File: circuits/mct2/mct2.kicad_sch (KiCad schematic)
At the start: 4 parts, among them J1 Bus_M.2_Socket_M, J2 Bus_M.2_Socket_E, U1 BQ25700A

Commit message: schem update July 19 2024
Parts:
- removed U1: BQ25700A, symbol mediacow:BQ25700A
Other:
- added sheet mct2_power (mct2_power.kicad_sch)
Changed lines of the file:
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@@
-		)
-	)
-	(wire
-		(pts
-			(xy 229.87 749.3) (xy 232.41 749.3)
-		)
-		(stroke
-			(width 0)
-			(type default)
 		)
 	)
@@
 		)
 	)
-	(global_label "PROCHOT"
-		(shape input)
-		(at 229.87 749.3 180)
-		(fields_autoplaced yes)
-		(effects
-			(font
-				(size 1.27 1.27)
-			)
-			(justify right)
-		)
-		(property "Intersheetrefs" "${INTERSHEET_REFS}"
-			(at 218.1157 749.3 0)
-			(effects
-				(font
-					(size 1.27 1.27)
-				)
-				(justify right)
-				(hide yes)
-			)
-		)
-	)
 	(global_label "AC_LRCLK"
 		(shape input)
@@
 				(justify left)
 				(hide yes)
-			)
-		)
-	)
-	(symbol
-		(lib_id "mediacow:BQ25700A")
-		(at 247.65 742.95 0)
-		(unit 1)
-		(exclude_from_sim no)
-		(in_bom yes)
-		(on_board yes)
-		(dnp no)
-		(property "Reference" "U1"
-			(at 236.22 720.344 0)
-			(effects
-				(font
-					(size 1.27 1.27)
-				)
-			)
-		)
-		(property "Value" "BQ25700A"
-			(at 243.332 720.344 0)
-			(effects
-				(font
-					(size 1.27 1.27)
-				)
-			)
-		)
-		(property "Footprint" ""
-			(at 241.3 727.71 0)
-			(effects
-				(font
-					(size 1.27 1.27)
-				)
-				(hide yes)
-			)
-		)
-		(property "Datasheet" ""
-			(at 241.3 727.71 0)
-			(effects
-				(font
-					(size 1.27 1.27)
-				)
-				(hide yes)
-			)
-		)
-		(property "Description" ""
-			(at 241.3 727.71 0)
-			(effects
-				(font
-					(size 1.27 1.27)
-				)
-				(hide yes)
-			)
-		)
-		(pin "32"
-		)
-		(pin "23"
-		)
-		(pin "25"
-		)
-		(pin "17"
-		)
-		(pin "22"
-		)
-		(pin "6"
-		)
-		(pin "31"
-		)
-		(pin "19"
-		)
-		(pin "29"
-		)
-		(pin "16"
-		)
-		(pin "26"
-		)
-		(pin "15"
-		)
-		(pin "1"
-		)
-		(pin "28"
-		)
-		(pin "11"
-		)
-		(pin "13"
-		)
-		(pin "9"
-		)
-		(pin "5"
-		)
-		(pin "12"
-		)
-		(pin "3"
-		)
-		(pin "8"
-		)
-		(pin "20"
-		)
-		(pin "21"
-		)
-		(pin "30"
-		)
-		(pin "4"
-		)
-		(pin "27"
-		)
-		(pin "10"
-		)
-		(pin "7"
-		)
-		(pin "2"
-		)
-		(pin "24"
-		)
-		(pin "18"
-		)
-		(pin "14"
-		)
-		(instances
-			(project "mct2"
-				(path "/0917e100-0497-47cd-9e32-3e43ad224d2b"
-					(reference "U1")
-					(unit 1)
-				)
 			)
 		)
@@
 				)
 			)
+		)
+	)
+	(sheet
+		(at 688.34 405.13)
+		(size 67.31 55.88)
+		(fields_autoplaced yes)
+		(stroke
+			(width 0.1524)
+			(type solid)
+		)
+		(fill
+			(color 0 0 0 0.0000)
+		)
+		(property "Sheetname" "mct2_power"
+			(at 688.34 404.4184 0)
+			(effects
+				(font
+					(size 1.27 1.27)
+				)
+				(justify left bottom)
+			)
+		)
+		(property "Sheetfile" "mct2_power.kicad_sch"
+			(at 688.34 461.5946 0)
+			(effects
+				(font
+					(size 1.27 1.27)
+				)
+				(justify left top)
+			)
+		)
+		(instances
+			(project "mct2"
+				(path "/0917e100-0497-47cd-9e32-3e43ad224d2b"
+					(page "3")
+				)
+			)

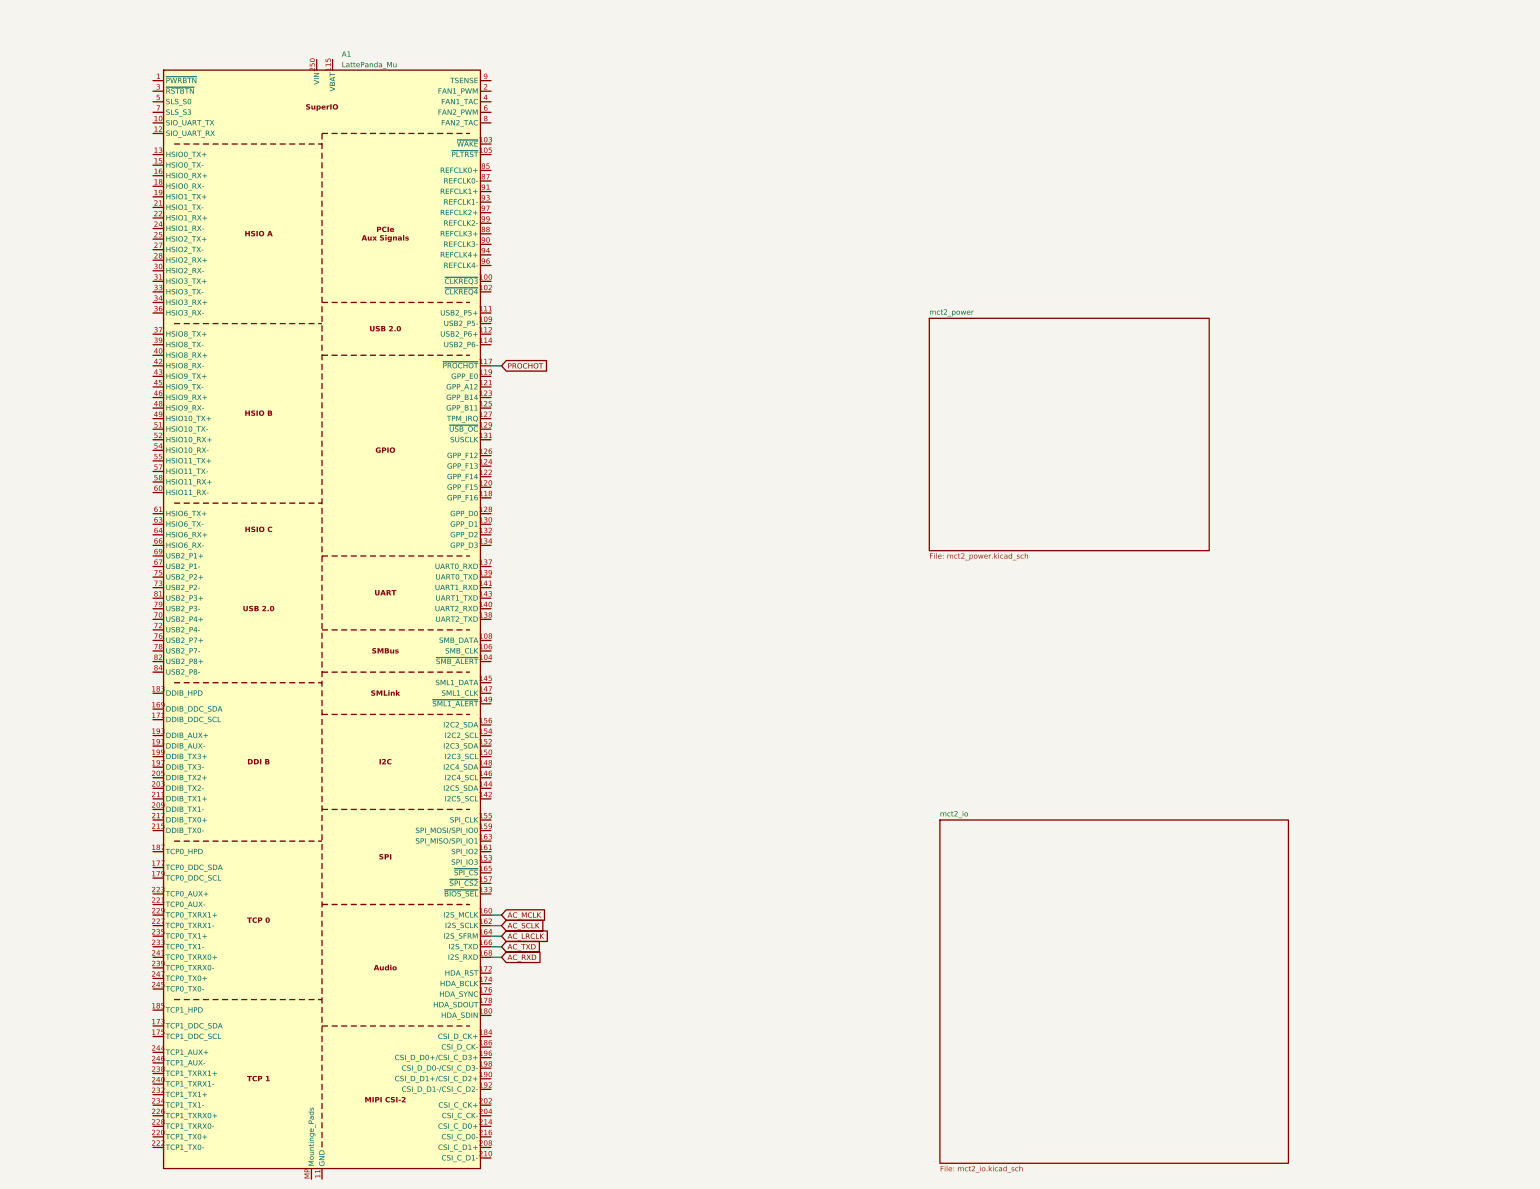
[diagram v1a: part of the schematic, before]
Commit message: July 21, 2024
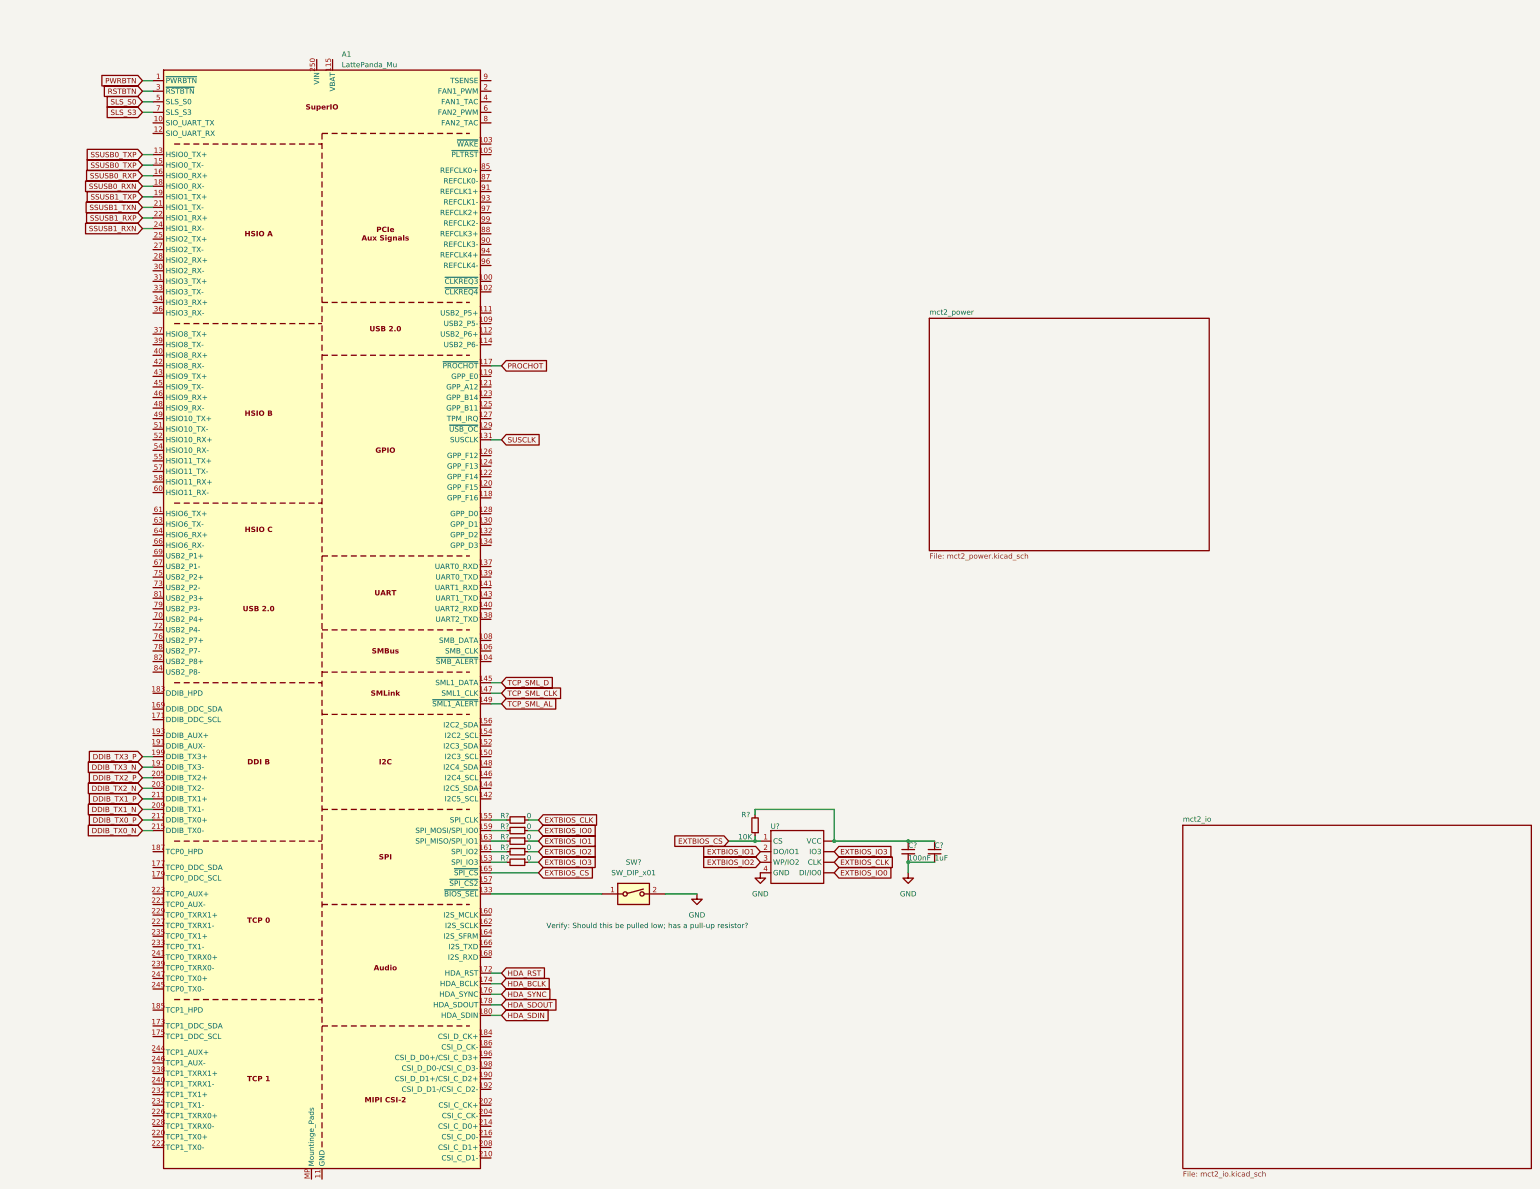
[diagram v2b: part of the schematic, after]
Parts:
- added C?: 1uF, symbol Device:C_Small
- added C?: 100nF, symbol Device:C_Small
- added R? (x5): 0, symbol Device:R_Small
- added R?: 10K, Resistor_SMD:R_0603_1608Metric, symbol Device:R_Small
- added SW?: SW_DIP_x01, symbol Switch:SW_DIP_x01
- added U?: ~, symbol mediacow:SPI_FLS_G6179-10
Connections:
- net PWRBTN: now reaches A1.1 (~{PWRBTN})
- net SSUSB0_TXP: now reaches A1.13 (HSIO0_TX+)
- net SSUSB0_TXP: now also A1.15 (HSIO0_TX-)
- net SUSCLK: now reaches A1.131 (SUSCLK)
- net at A1.133 (~{BIOS_SEL}): now also SW?.1
- net TCP_SML_D: now reaches A1.145 (SML1_DATA)
- net TCP_SML_CLK: now reaches A1.147 (SML1_CLK)
- net TCP_SML_AL: now reaches A1.149 (~{SML1_ALERT})
- net at A1.153 (SPI_IO3): now also R?.2
- net at A1.155 (SPI_CLK): now also R?.2
- net at A1.159 (SPI_MOSI/SPI_IO0): now also R?.2
- net SSUSB0_RXP: now reaches A1.16 (HSIO0_RX+)
- net at A1.161 (SPI_IO2): now also R?.2
- net at A1.163 (SPI_MISO/SPI_IO1): now also R?.2
- net EXTBIOS_CS: now reaches A1.165 (~{SPI_CS})
- net EXTBIOS_CS: now also R?.1, U?.1 (CS)
- net HDA_RST: now reaches A1.172 (HDA_RST)
- net HDA_BCLK: now reaches A1.174 (HDA_BCLK)
- net HDA_SYNC: now reaches A1.176 (HDA_SYNC)
- net HDA_SDOUT: now reaches A1.178 (HDA_SDOUT)
- net SSUSB0_RXN: now reaches A1.18 (HSIO0_RX-)
- net HDA_SDIN: now reaches A1.180 (HDA_SDIN)
- net SSUSB1_TXP: now reaches A1.19 (HSIO1_TX+)
- net DDIB_TX3_N: now reaches A1.197 (DDIB_TX3-)
- net DDIB_TX3_P: now reaches A1.199 (DDIB_TX3+)
- net DDIB_TX2_N: now reaches A1.203 (DDIB_TX2-)
- net DDIB_TX2_P: now reaches A1.205 (DDIB_TX2+)
- net DDIB_TX1_N: now reaches A1.209 (DDIB_TX1-)
- net SSUSB1_TXN: now reaches A1.21 (HSIO1_TX-)
- net DDIB_TX1_P: now reaches A1.211 (DDIB_TX1+)
- net DDIB_TX0_N: now reaches A1.215 (DDIB_TX0-)
- net DDIB_TX0_P: now reaches A1.217 (DDIB_TX0+)
- net SSUSB1_RXP: now reaches A1.22 (HSIO1_RX+)
- net SSUSB1_RXN: now reaches A1.24 (HSIO1_RX-)
- net RSTBTN: now reaches A1.3 (~{RSTBTN})
- net SLS_S0: now reaches A1.5 (SLS_S0)
- net SLS_S3: now reaches A1.7 (SLS_S3)
- net AC_LRCLK: no longer names the net of A1.164 (I2S_SFRM)
- net AC_MCLK: no longer names the net of A1.160 (I2S_MCLK)
- net AC_RXD: no longer names the net of A1.168 (I2S_RXD)
- net AC_SCLK: no longer names the net of A1.162 (I2S_SCLK)
- net AC_TXD: no longer names the net of A1.166 (I2S_TXD)
- new net: C?.1, C?.1, R?.2, U?. (VCC)
- new net EXTBIOS_CLK: R?.1, U?. (VCC)
- new net EXTBIOS_IO0: R?.1, U?. (VCC)
- new net EXTBIOS_IO1: R?.1, U?.2 (DO/IO1)
- new net EXTBIOS_IO2: R?.1, U?.3 (WP/IO2)
- new net EXTBIOS_IO3: R?.1, U?. (VCC)
- new net GND: C?.2, C?.2, SW?.2, U?.4 (GND)
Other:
- note added: "Verify: Should this be pulled low; has a pull-up resistor?"
